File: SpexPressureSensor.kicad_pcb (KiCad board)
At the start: 2 copper layers, 51 x 51 mm, 68 parts, among them J1 3PinJumper, J2 edgeMountSMA, P1 CONN_6, P2 NICHROME, P3 TC2030-CTX, Q1 IRLL3303PbF, Q2 MOS_N_numbered, Q3 MOS_N_numbered, Q4 MMBT4403, Q5 MOS_N_numbered, Q6 MOS_N_numbered, U1 ST1480ABDR, U2 TPS769XX, U3 MKL03ZxxVFG4, U4 BMP180, U5 MMA8653FC, U6 SI5351A, U7 LT6105, X1 NX3225GA

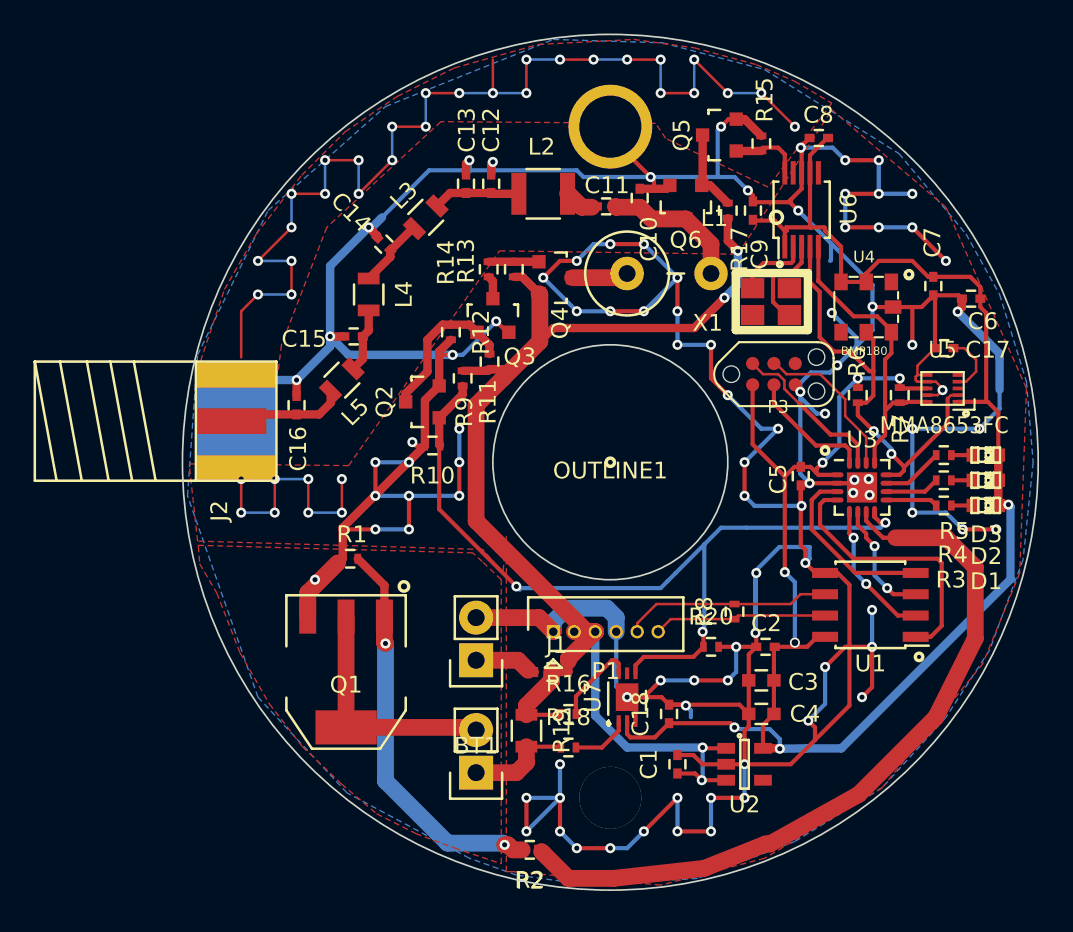
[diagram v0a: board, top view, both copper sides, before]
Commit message: Realized the board was tooooo big.
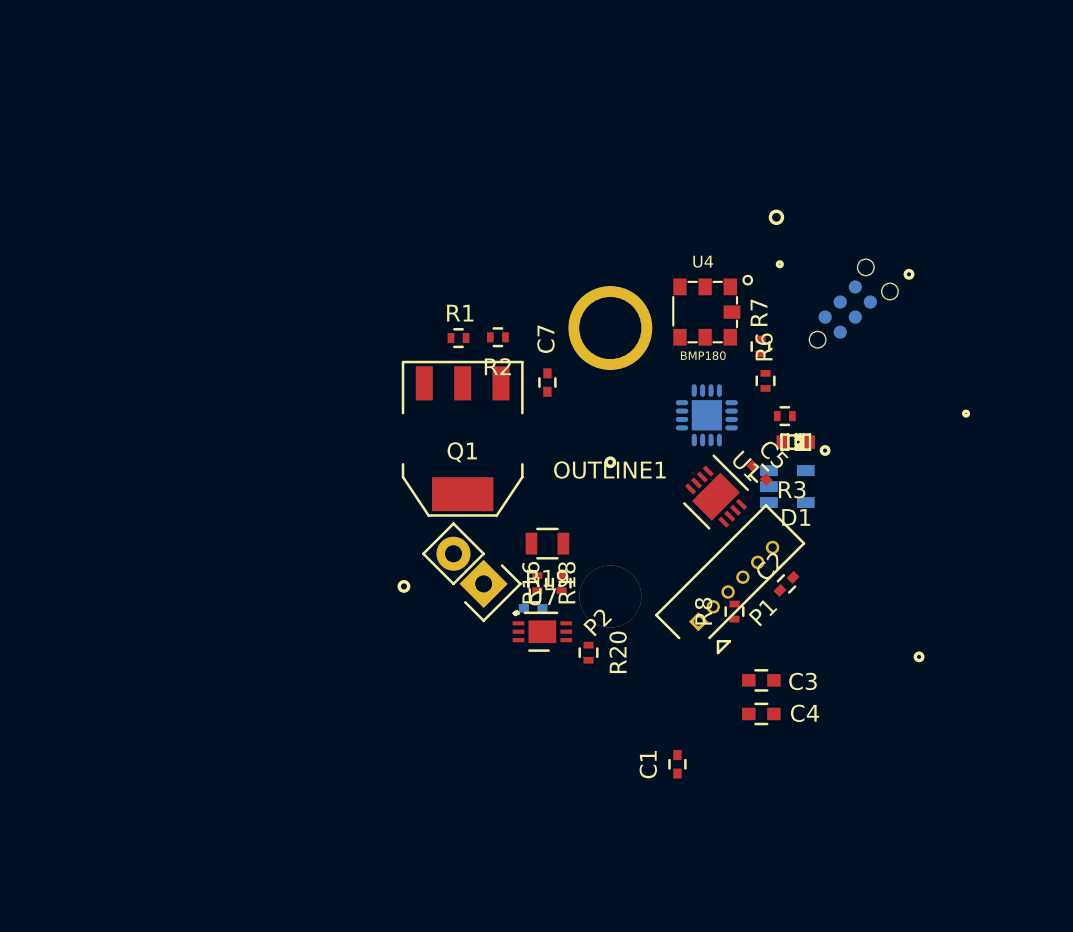
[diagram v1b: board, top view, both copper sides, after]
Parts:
- removed BT1: BATTERY, Pin_Headers:Pin_Header_Straight_1x02
- removed C10: 47p, Capacitors_SMD:C_0402
- removed C11: 100p, Capacitors_SMD:C_0402
- removed C12: 56p, Capacitors_SMD:C_0402
- removed C13, C16: 150p, Capacitors_SMD:C_0402
- removed C14, C15: 220p, Capacitors_SMD:C_0402
- removed C17, C6, C8: 1uf, Capacitors_SMD:C_0402
- removed C9: .47uf, Capacitors_SMD:C_0402
- removed D2, D3: LED, LEDs:LED-0603
- removed G***: LOGO, spexLogo:logoBig
- removed J1: 3PinJumper, solderJmp:3solderJmp
- removed J2: edgeMountSMA, edgeSMA:EdgeSMA
- removed L1: INDUCTOR_SMALL, Resistors_ThroughHole:Resistor_Vertical_RM5mm
- removed L2: 4uh, Resistors_SMD:R_1210
- removed L3, L5: 390n, Resistors_SMD:R_0805
- removed L4: 470n, Resistors_SMD:R_0805
- removed Q2, Q3, Q5, Q6: MOS_N_numbered, Housings_SOT-23_SOT-143_TSOT-6:SOT-23
- removed Q4: MMBT4403, Housings_SOT-23_SOT-143_TSOT-6:SOT-23
- removed R10: DNP, Resistors_SMD:R_0402
- removed R11: 2K, Resistors_SMD:R_0402
- removed R12, R9: 10K, Resistors_SMD:R_0402
- removed R13, R14: 1K, Resistors_SMD:R_0402
- removed R15: 2000, Resistors_SMD:R_0402
- removed R17: R, Resistors_SMD:R_0402
- removed R4, R5: 100, Resistors_SMD:R_0402
- removed U5: MMA8653FC, MMA8653FC:MMA8653FCR1
- removed U6: SI5351A, Housings_SSOP:MSOP-10_3x3mm_Pitch0.5mm
- removed X1: NX3225GA, NX3225GA:NX3225GA
- C18, P3, U2, U3: moved to B.Cu
- U1: footprint Housings_SOIC:SOIC-8_3.9x4.9mm_Pitch1.27mm -> Housings_DFN_QFN:DFN-8-1EP_3x3mm_Pitch0.5mm
- moved R2 30.6 mm to (113.3, 57.5)
- moved C7 23.7 mm to (116.2, 60.2)
- moved U2 16.7 mm to (130.6, 66.5)
- moved Q1 15.5 mm to (111.2, 63.6)
- moved R1 14.6 mm to (111.0, 57.6)
- moved D1 11.9 mm to (131.1, 63.8)
- moved P2 11.3 mm to (112.5, 72.2), turned to 225 degrees
- moved U1 11.2 mm to (126.3, 67.0), turned to 315 degrees
- moved R19 11.2 mm to (116.2, 69.8), turned to 180 degrees
- moved R3 10.9 mm to (130.4, 62.2)
- moved C18 10.3 mm to (115.4, 73.7), turned to 0 degrees
- moved U3 10.2 mm to (125.8, 62.2), turned to 180 degrees
- moved R18 9.97 mm to (115.7, 72.2), turned to 270 degrees
- moved U4 9.60 mm to (125.7, 56.0)
- moved R7 8.79 mm to (128.9, 58.1), turned to 90 degrees
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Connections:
- net /Beacon/KEY renamed /NichromeI
- net /Beacon/SCL renamed Net-(R6-Pad2)
- net /Beacon/SDA renamed Net-(R7-Pad2)
- C1 pad 1: /Beacon/12V -> /VInput
- P1 pad 2: /Beacon/12V -> /VInput
- P1 pad 3: /Beacon/12V -> /VInput
- R16 pad 1: Net-(J1-Pad2) -> /VInput
- R19 pad 1: Net-(J1-Pad2) -> /VInput
- U2 pad 1: /Beacon/12V -> /VInput
- U2 pad 3: /Beacon/12V -> /VInput
- U3 pad 10: Net-(R4-Pad2) -> (no net)
- U3 pad 11: Net-(R5-Pad2) -> (no net)
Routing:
- net GND: track 403.1 -> 0.00 mm, vias 102 -> 0
- net +3.3V: track 120.4 -> 0.00 mm, vias 8 -> 0
- net /Beacon/12V: track 74.2 -> 0.00 mm, vias 4 -> 0
- net (no net): track 63.5 -> 0.00 mm, vias 28 -> 0
- net /NichromeI: track 51.1 -> 0.00 mm, vias 3 -> 0
- net Net-(R2-Pad1): track 45.2 -> 0.00 mm
- net Net-(R6-Pad2): track 27.0 -> 0.00 mm, vias 2 -> 0
- net Net-(Q1-Pad1): track 23.8 -> 0.00 mm, vias 2 -> 0
- net Net-(R7-Pad2): track 18.7 -> 0.00 mm
- net Net-(P2-Pad2): track 16.4 -> 0.00 mm
- net Net-(U1-Pad1): track 16.1 -> 0.00 mm
- net Net-(P1-Pad5): track 12.4 -> 0.00 mm
- net Net-(U1-Pad4): track 10.8 -> 0.00 mm
- net Net-(P1-Pad6): track 10.4 -> 0.00 mm
- net /SWDIO: track 9.65 -> 0.00 mm
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- removed copper zone on B.Cu, net GND
- removed copper zone on F.Cu, net GND
- removed copper zone on F.Cu, net Net-(P2-Pad2)
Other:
- board outline removed
